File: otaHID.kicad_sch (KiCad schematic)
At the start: 25 parts, among them J1 USB_A, J2 A1001WR-S-2P, J3 STM32_Debug, SW1 TVAF06-A020B-R, U1 NJW4183U3, U2 LXES11DAA2-135, U3 STM32L4P5CGT6, U4 RN4020, U5 TLP172AM, Y1 12MHz

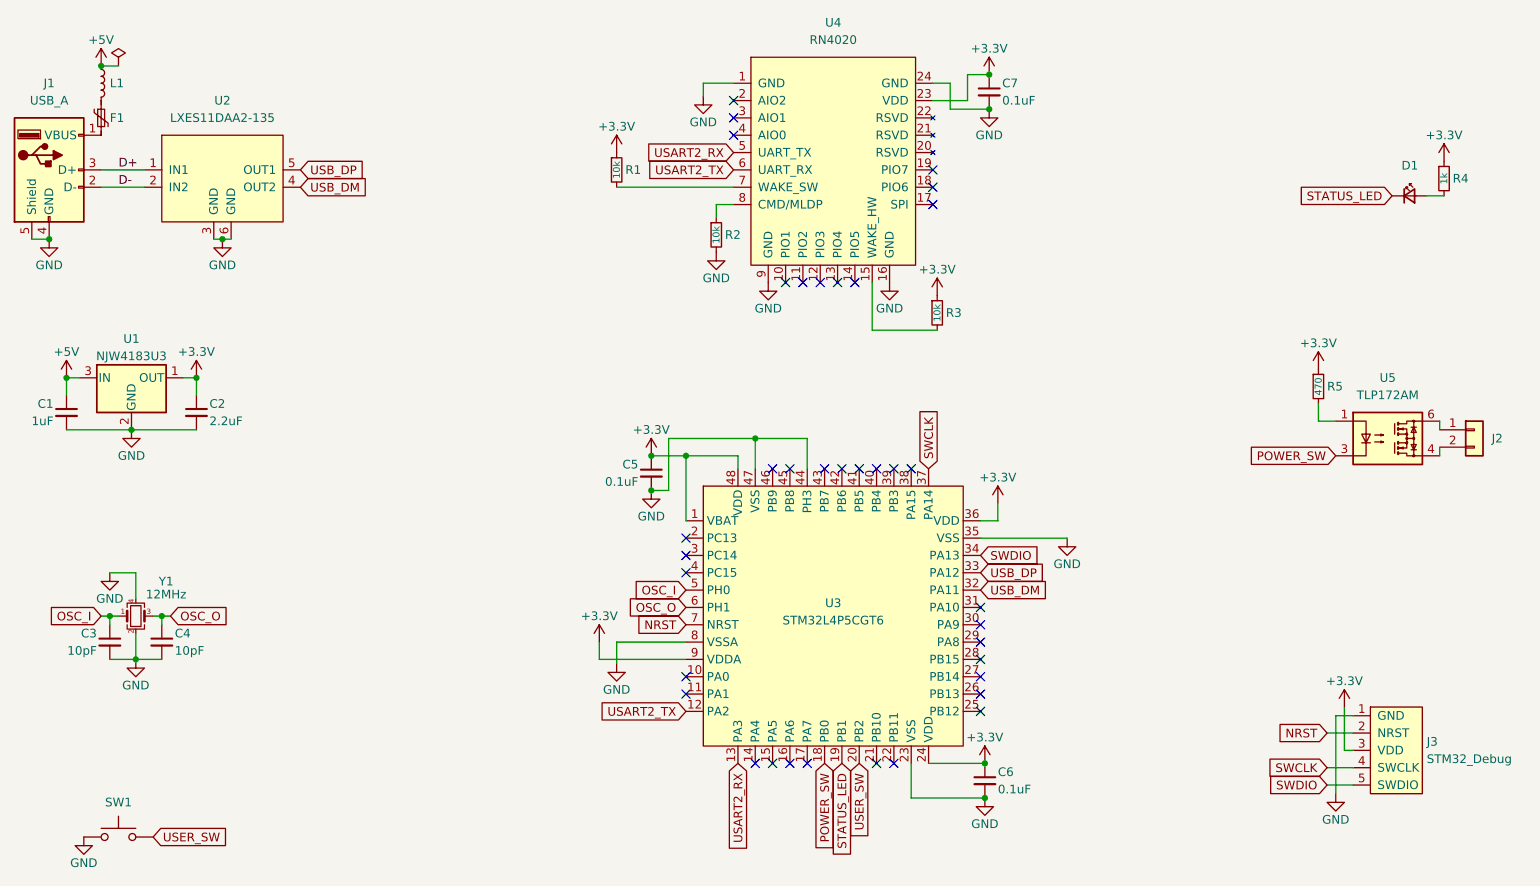
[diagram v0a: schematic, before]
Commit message: 基盤v2.0
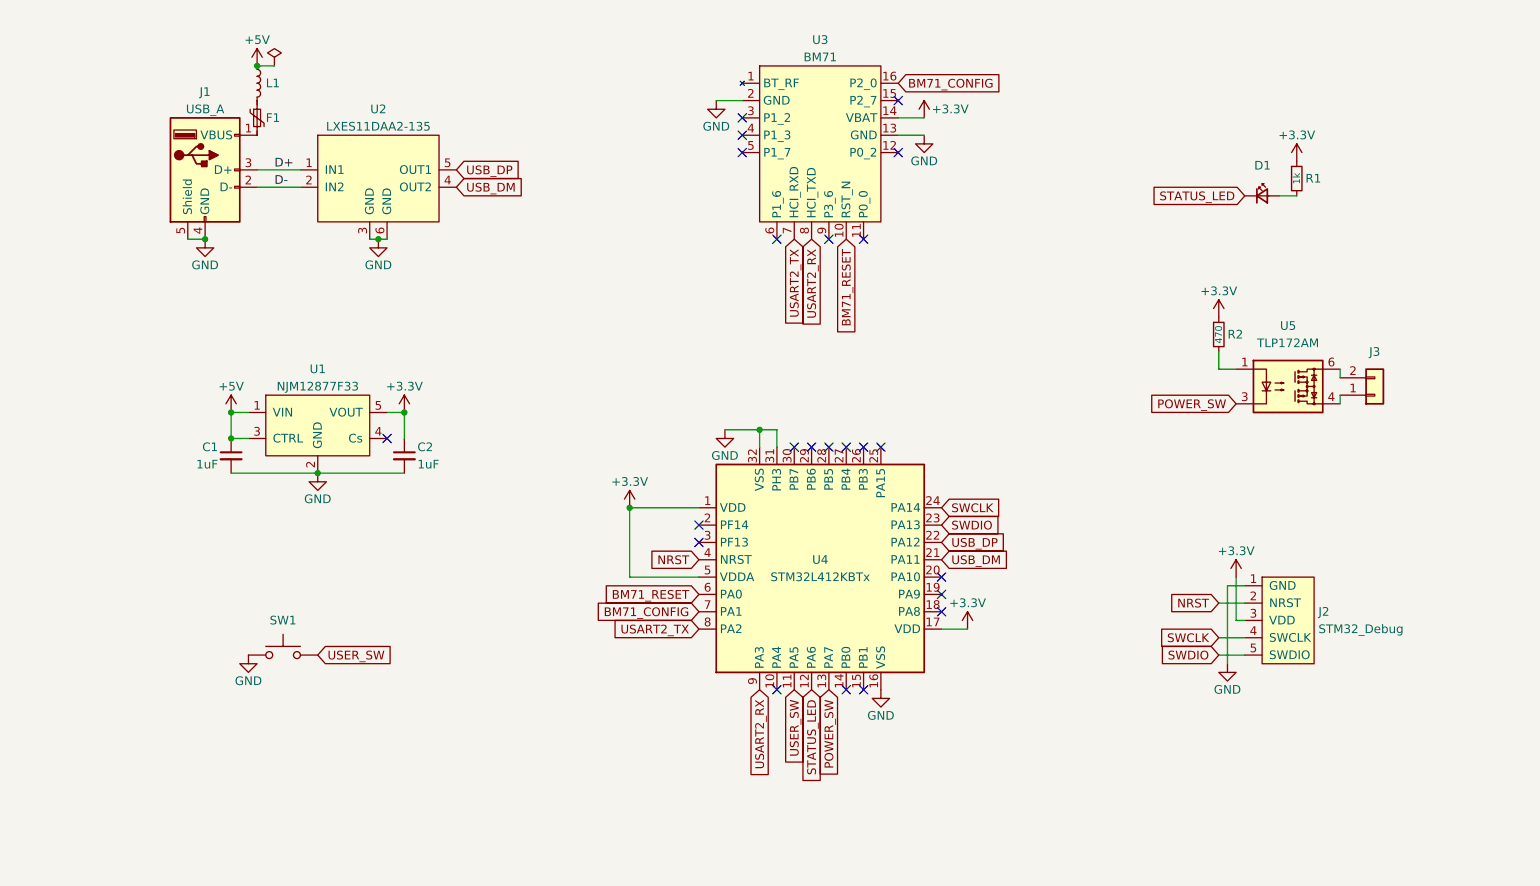
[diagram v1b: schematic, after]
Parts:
- removed C3, C4: 10pF, otaHID:1005Metric, symbol Device:C_Small
- removed C5, C6, C7: 0.1uF, otaHID:1608Metric, symbol Device:C_Small
- removed R1, R2, R3: 10k, otaHID:1608Metric, symbol Device:R_Small
- removed U1: NJW4183U3, otaHID:SOT-89-3, symbol otaHID:NJW4183U3
- removed U3: STM32L4P5CGT6, otaHID:LQFP-48_7x7mm_P0.5mm_FusionPCB, symbol otaHID:STM32L4P5CGT6
- removed U4: RN4020, otaHID:RN4020, symbol otaHID:RN4020
- removed Y1: 12MHz, otaHID:Crystal_SMD_3225-4Pin_3.2x2.5mm_HandSoldering, symbol Device:Crystal_GND24_Small
- added U1: NJM12877F33, otaHID:SOT-23-5, symbol otaHID:NJM12877F33
- added U3: BM71, otaHID:BM71, symbol otaHID:BM71
- added U4: STM32L412KBTx, otaHID:QFN-32-1EP_5x5mm_P0.5mm_EP3.3x3.3mm, symbol otaHID:STM32L412KBTx
- C2: value 2.2uF -> 1uF
- SW1: footprint otaHID:SW_TVAF06 -> otaHID:SideSW_THAF01-NC-R
- renumbered J3 to J2, J2 to J3, R4 to R1, R5 to R2
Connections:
- net +5V: now also U1.1 (VIN), U1.3 (CTRL)
- net GND: now also SW1.2, U1.2 (GND), U3.13 (GND), U3.2 (GND), U4.16 (VSS), U4.31 (PH3), U4.32 (VSS); no longer SW1.1
- net NRST: now also U4.4 (NRST)
- net POWER_SW: now also U4.13 (PA7)
- net STATUS_LED: now also U4.12 (PA6)
- net SWCLK: now also U4.24 (PA14)
- net SWDIO: now also U4.23 (PA13)
- net USART2_RX: now also U3.8 (HCI_TXD), U4.9 (PA3)
- net USART2_TX: now also U3.7 (HCI_RXD), U4.8 (PA2)
- net USB_DM: now also U4.21 (PA11)
- net USB_DP: now also U4.22 (PA12)
- net USER_SW: now also SW1.1, U4.11 (PA5); no longer SW1.2
- net at J3.1 (Pin_1): now also U5.4; no longer U5.6
- net at J3.2 (Pin_2): now also U5.6; no longer U5.4
- net +3V3 renamed +3.3V
- net +3.3V: now also U1.5 (VOUT), U3.14 (VBAT), U4.1 (VDD), U4.17 (VDD), U4.5 (VDDA)
- new net BM71_CONFIG: U3.16 (P2_0), U4.7 (PA1)
- new net BM71_RESET: U3.10 (RST_N), U4.6 (PA0)
- no-connect marks 37 -> 23
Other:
- moved on the sheet: C1, C2, D1, F1, J1, J2, J3, L1, R1, R2, SW1, U2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

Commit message: 基板 V2.1
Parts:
- C1, C2, R1, R2: footprint otaHID:1608Metric -> otaHID:1005Metric
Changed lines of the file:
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@@
       (effects (font (size 1.016 1.016)))
     )
-    (property "Footprint" "otaHID:1608Metric" (id 2) (at 222.25 50.8 0)
+    (property "Footprint" "otaHID:1005Metric" (id 2) (at 222.25 50.8 0)
       (effects (font (size 1.27 1.27)) hide)
     )
@@
       (effects (font (size 1.27 1.27)) (justify left))
     )
-    (property "Footprint" "otaHID:1608Metric" (id 2) (at 91.44 91.44 0)
+    (property "Footprint" "otaHID:1005Metric" (id 2) (at 91.44 91.44 0)
       (effects (font (size 1.27 1.27)) hide)
     )
@@
       (effects (font (size 1.016 1.016)))
     )
-    (property "Footprint" "otaHID:1608Metric" (id 2) (at 210.82 73.66 0)
+    (property "Footprint" "otaHID:1005Metric" (id 2) (at 210.82 73.66 0)
       (effects (font (size 1.27 1.27)) hide)
     )
@@
       (effects (font (size 1.27 1.27)) (justify left))
     )
-    (property "Footprint" "otaHID:1608Metric" (id 2) (at 66.04 91.44 0)
+    (property "Footprint" "otaHID:1005Metric" (id 2) (at 66.04 91.44 0)
       (effects (font (size 1.27 1.27)) hide)
     )
@@
     )
     (path "/d499b390-4b94-487e-8623-92901e75e504"
-      (reference "C1") (unit 1) (value "1uF") (footprint "otaHID:1608Metric")
+      (reference "C1") (unit 1) (value "1uF") (footprint "otaHID:1005Metric")
     )
     (path "/a4db60fc-1523-4e61-8459-c8b02fdf3d76"
-      (reference "C2") (unit 1) (value "1uF") (footprint "otaHID:1608Metric")
+      (reference "C2") (unit 1) (value "1uF") (footprint "otaHID:1005Metric")
     )
     (path "/ecc7aa79-03bd-4a5d-9770-720de9966d4d"
@@
     )
     (path "/4650ece2-e1f8-4b4f-8fa2-6a844fad8b1d"
-      (reference "R1") (unit 1) (value "1k") (footprint "otaHID:1608Metric")
+      (reference "R1") (unit 1) (value "1k") (footprint "otaHID:1005Metric")
     )
     (path "/ca33f7e4-ee7d-45b9-84d5-8203e17df579"
-      (reference "R2") (unit 1) (value "470") (footprint "otaHID:1608Metric")
+      (reference "R2") (unit 1) (value "470") (footprint "otaHID:1005Metric")
     )
     (path "/6a799451-a531-4b03-86b8-defa29791348"
